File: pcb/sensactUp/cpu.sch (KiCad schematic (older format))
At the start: 15 parts, among them P7 USB, U3 STM32F072C8Tx, Y1 Crystal_GND24

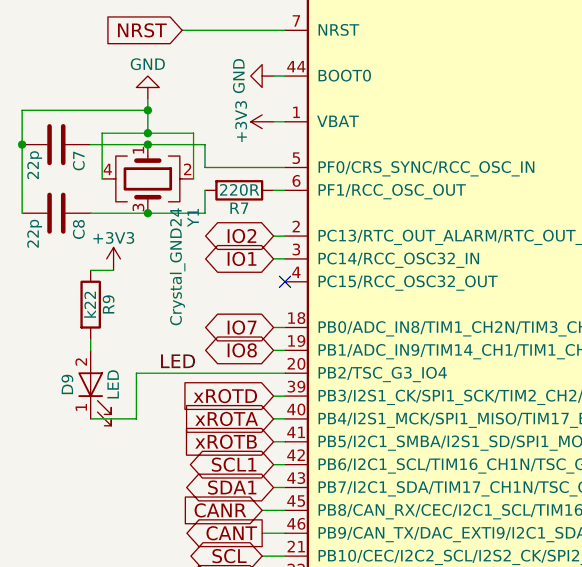
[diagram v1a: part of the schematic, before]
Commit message: Unspecified
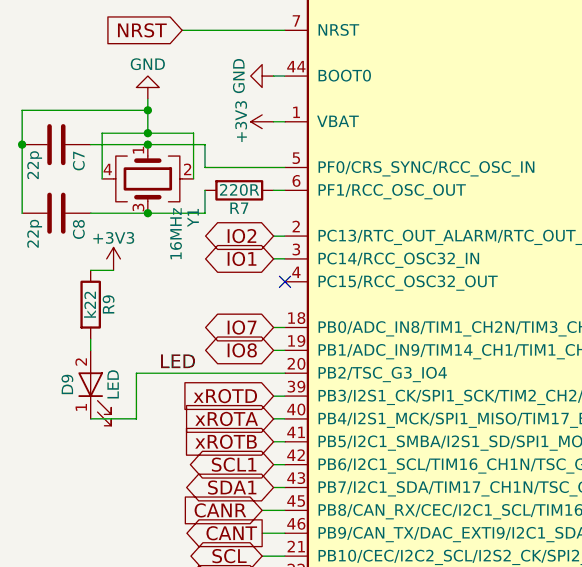
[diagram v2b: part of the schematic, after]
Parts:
- Y1: value Crystal_GND24 -> 16MHz
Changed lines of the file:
@@
 P 1100 2850
 F 0 "Y1" H 1225 3050 50  0000 L CNN
-F 1 "Crystal_GND24" H 1225 2975 50  0000 L CNN
+F 1 "16MHz" H 1225 2975 50  0000 L CNN
 F 2 "sensact:quartz3225" H 1100 2850 50  0001 C CNN
 F 3 "" H 1100 2850 50  0000 C CNN

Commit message: WHS lIb
WHS lIb
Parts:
- C15, C16, C17, C18, C19, C20, C7, C8: symbol C -> Device:C
- D9: symbol LED -> Device:LED
- FB1: symbol FILTER -> sensactUp-rescue:FILTER
- P7: symbol CONN_01X03 -> sensactUp-rescue:CONN_01X03
- R7, R9: symbol R -> Device:R
- U3: symbol STM32F072C8Tx -> sensactUp-rescue:STM32F072C8Tx
- Y1: symbol Crystal_GND24 -> Device:Crystal_GND24
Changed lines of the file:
@@
-EESchema Schematic File Version 2
-LIBS:power
-LIBS:device
-LIBS:transistors
-LIBS:conn
-LIBS:linear
-LIBS:regul
-LIBS:74xx
-LIBS:cmos4000
-LIBS:adc-dac
-LIBS:memory
-LIBS:xilinx
-LIBS:microcontrollers
-LIBS:dsp
-LIBS:microchip
-LIBS:analog_switches
-LIBS:motorola
-LIBS:texas
-LIBS:intel
-LIBS:audio
-LIBS:interface
-LIBS:digital-audio
-LIBS:philips
-LIBS:display
-LIBS:cypress
-LIBS:siliconi
-LIBS:opto
-LIBS:atmel
-LIBS:contrib
-LIBS:valves
-LIBS:stm32
-LIBS:switches
-LIBS:relays
-LIBS:sensact
-LIBS:mechanical
+EESchema Schematic File Version 4
 LIBS:sensactUp-cache
-EELAYER 25 0
+EELAYER 26 0
 EELAYER END
 $Descr A4 11693 8268
@@
 $EndDescr
 $Comp
-L STM32F072C8Tx U3
+L sensactUp-rescue:STM32F072C8Tx U3
 U 1 1 58B753F2
 P 5500 3600
@@
 $EndComp
 $Comp
-L C C19
+L Device:C C19
 U 1 1 58B754C8
 P 4700 1300
@@
 $EndComp
 $Comp
-L C C20
+L Device:C C20
 U 1 1 58B754E7
 P 4900 1300
@@
 $EndComp
 $Comp
-L C C15
+L Device:C C15
 U 1 1 58B75545
 P 3250 1300
@@
 $EndComp
 $Comp
-L C C18
+L Device:C C18
 U 1 1 58B7557A
 P 3850 1300
@@
 $EndComp
 $Comp
-L C C17
+L Device:C C17
 U 1 1 58B755AD
 P 3650 1300
@@
 $EndComp
 $Comp
-L C C16
+L Device:C C16
 U 1 1 58B755D0
 P 3450 1300
@@
 $EndComp
 $Comp
-L +3V3 #PWR057
+L power:+3V3 #PWR057
 U 1 1 58B75879
 P 5350 1650
@@
 $EndComp
 $Comp
-L +3V3 #PWR058
+L power:+3V3 #PWR058
 U 1 1 58B7589B
 P 5600 1650
@@
 	5400 1650 5400 1700
 Wire Wire Line
-	5300 1650 5400 1650
+	5300 1650 5350 1650
 Wire Wire Line
 	5300 1700 5300 1650
 Connection ~ 5350 1650
 $Comp
-L +3.3VA #PWR059
+L power:+3.3VA #PWR059
 U 1 1 58B75979
 P 5500 1450
@@
 Connection ~ 4700 1150
 $Comp
-L +3.3VA #PWR060
+L power:+3.3VA #PWR060
 U 1 1 58B759CE
 P 4800 950
@@
 Connection ~ 4800 1150
 Wire Wire Line
-	3250 1150 3950 1150
+	3250 1150 3450 1150
 Connection ~ 3850 1150
 Connection ~ 3650 1150
 Connection ~ 3450 1150
 $Comp
-L +3V3 #PWR061
+L power:+3V3 #PWR061
 U 1 1 58B75AF2
 P 3550 1100
@@
 Connection ~ 3550 1150
 Wire Wire Line
-	3250 1450 4900 1450
+	3250 1450 3450 1450
 Connection ~ 4700 1450
 Connection ~ 3850 1450
@@
 Connection ~ 3450 1450
 $Comp
-L GND #PWR062
+L power:GND #PWR062
 U 1 1 58B75BBF
 P 3550 1500
@@
 Connection ~ 3550 1450
 $Comp
-L GND #PWR063
+L power:GND #PWR063
 U 1 1 58B75C63
 P 5450 5450
@@
 $EndComp
 Wire Wire Line
-	5300 5450 5600 5450
+	5300 5450 5400 5450
 Wire Wire Line
 	5600 5450 5600 5400
@@
 Connection ~ 5400 5450
 $Comp
-L FILTER FB1
+L sensactUp-rescue:FILTER FB1
 U 1 1 58B76153
 P 4300 1150
@@
 $EndComp
 Wire Wire Line
-	4650 1150 4900 1150
+	4650 1150 4700 1150
 Text GLabel 1250 2200 0    60   Input ~ 0
 NRST
@@
 	1700 2200 1250 2200
 $Comp
-L GND #PWR064
+L power:GND #PWR064
 U 1 1 58B775D8
 P 1650 2400
@@
 $EndComp
 $Comp
-L +3V3 #PWR065
+L power:+3V3 #PWR065
 U 1 1 58B775FC
 P 1650 2600
@@
 	1700 2600 1650 2600
 $Comp
-L Crystal_GND24 Y1
+L Device:Crystal_GND24 Y1
 U 1 1 58B7767E
 P 1100 2850
@@
 	1350 2700 1350 2800
 Wire Wire Line
-	850  2700 1350 2700
-Wire Wire Line
-	850  3000 1350 3000
+	850  2700 1100 2700
+Wire Wire Line
+	850  3000 1100 3000
 Wire Wire Line
 	1350 3000 1350 2900
@@
 	1300 2650 1300 2850
 Wire Wire Line
-	900  2650 1300 2650
+	900  2650 1100 2650
 Wire Wire Line
 	900  2650 900  2850
 $Comp
-L GND #PWR066
+L power:GND #PWR066
 U 1 1 58B7775E
 P 1100 2500
@@
 $EndComp
 Wire Wire Line
-	1100 2500 1100 2650
+	1100 2500 1100 2550
 Connection ~ 1100 2650
 $Comp
-L R R7
+L Device:R R7
 U 1 1 58B777BB
 P 1500 2900
@@
 	1350 2800 1700 2800
 $Comp
-L C C7
+L Device:C C7
 U 1 1 58B779D4
 P 700 2700
@@
 $EndComp
 $Comp
-L C C8
+L Device:C C8
 U 1 1 58B77A09
 P 700 3000
@@
 Connection ~ 1100 3000
 Wire Wire Line
-	550  2550 550  3000
+	550  2550 550  2700
 Wire Wire Line
 	550  2550 1100 2550
@@
 	1700 4400 1600 4400
 $Comp
-L GND #PWR067
+L power:GND #PWR067
 U 1 1 58B845F6
 P 10000 4800
@@
 	1700 4200 1650 4200
 $Comp
-L PWR_FLAG #FLG068
+L power:PWR_FLAG #FLG068
 U 1 1 58BB5186
 P 4900 1100
@@
 	1700 3200 1650 3200
 $Comp
-L R R9
+L Device:R R9
 U 1 1 595FEA9F
 P 850 3400
@@
 $EndComp
 $Comp
-L LED D9
+L Device:LED D9
 U 1 1 595FEC87
 P 850 3750
@@
 	850  3550 850  3600
 $Comp
-L +3V3 #PWR069
+L power:+3V3 #PWR069
 U 1 1 595FEDC0
 P 950 3250
@@
 LED
 $Comp
-L CONN_01X03 P7
+L sensactUp-rescue:CONN_01X03 P7
 U 1 1 59694EB9
 P 10250 4700
@@
 	10050 4800 10000 4800
 NoConn ~ 1700 3300
+Wire Wire Line
+	5350 1650 5400 1650
+Wire Wire Line
+	4700 1150 4800 1150
+Wire Wire Line
+	4800 1150 4900 1150
+Wire Wire Line
+	3850 1150 3950 1150
+Wire Wire Line
+	3650 1150 3850 1150
+Wire Wire Line
+	3450 1150 3550 1150
+Wire Wire Line
+	3550 1150 3650 1150
+Wire Wire Line
+	4700 1450 4900 1450
+Wire Wire Line
+	3850 1450 4700 1450
+Wire Wire Line
+	3650 1450 3850 1450
+Wire Wire Line
+	3450 1450 3550 1450
+Wire Wire Line
+	3550 1450 3650 1450
+Wire Wire Line
+	5500 5450 5600 5450
+Wire Wire Line
+	5450 5450 5500 5450
+Wire Wire Line
+	5400 5450 5450 5450
+Wire Wire Line
+	1100 2650 1300 2650
+Wire Wire Line
+	1100 2700 1350 2700
+Wire Wire Line
+	1100 3000 1350 3000
+Wire Wire Line
+	1100 2550 1100 2650
+Wire Wire Line
+	550  2700 550  3000
 $EndSCHEMATC
